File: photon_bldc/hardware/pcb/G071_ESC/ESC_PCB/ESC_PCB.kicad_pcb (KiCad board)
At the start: 6 copper layers, 12 x 32 mm, 65 parts, among them J2 Plus, J3 Minus, Q1 NMOS, Q2 NMOS, Q3 NMOS, Q4 NMOS, Q5 NMOS, Q6 NMOS, U1 STM32G071GBUx, U4 L78L06_SOT89

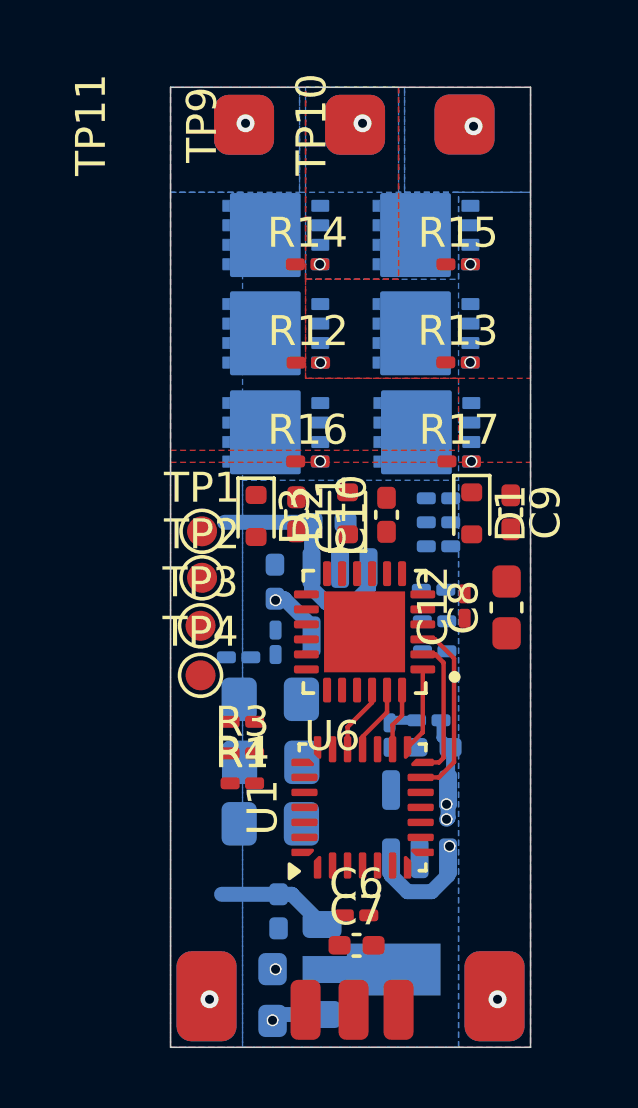
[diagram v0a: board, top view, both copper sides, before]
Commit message: ghjhbk
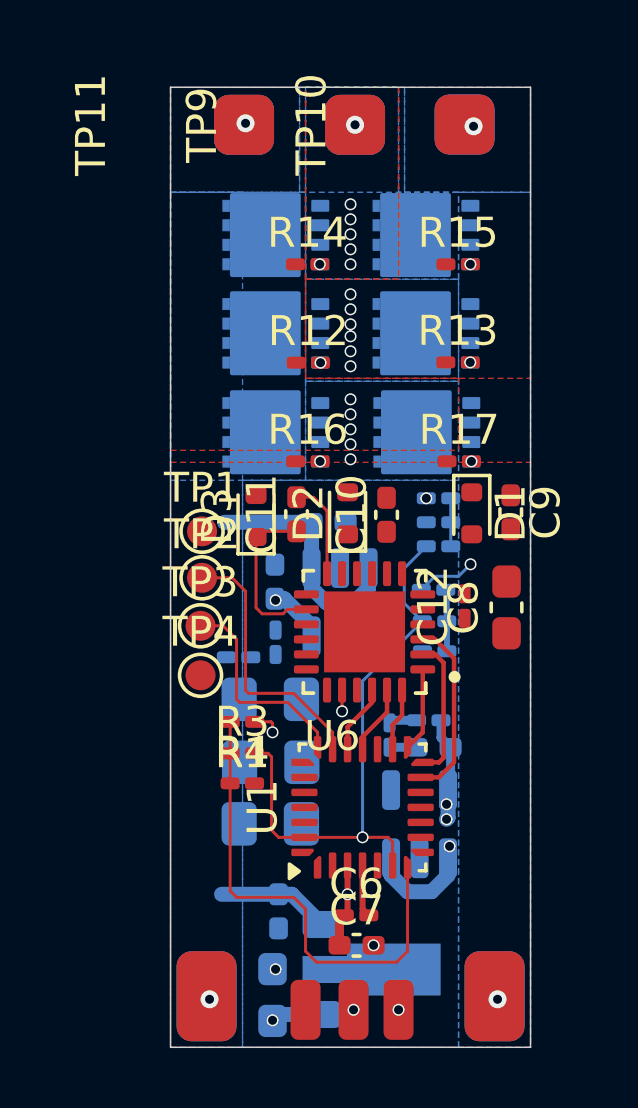
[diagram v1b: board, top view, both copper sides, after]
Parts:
- turned C11 to 90 degrees
- turned D3 to 90 degrees
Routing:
- net PHASE_C: track 0.00 -> 25.0 mm, vias 1 -> 7
- net BEMF_REF: track 0.00 -> 19.1 mm, vias 0 -> 1
- net BEMF_A: track 0.00 -> 16.3 mm
- net PHASE_A: track 0.00 -> 16.0 mm, vias 1 -> 7
- net PHASE_B: track 0.00 -> 13.1 mm, vias 1 -> 8
- net SWDIO: track 0.00 -> 8.98 mm
- net Net-(D1-K): track 0.00 -> 8.24 mm, vias 0 -> 1
- net SWCLK: track 0.00 -> 7.05 mm
- net Net-(D3-K): track 0.00 -> 5.61 mm
- net Net-(U6-VS3): track 0.00 -> 3.30 mm
- net +3.3V: track 3.53 -> 6.30 mm, vias 2 -> 3
- net GND: track 0.00 -> 2.65 mm, vias 2 -> 4
- net BEMF_C: track 0.00 -> 2.07 mm
- net BEMF_B: track 0.00 -> 1.60 mm
- net +5V: vias 1 -> 2
- added copper zone on In3.Cu, net +3.3V

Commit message: dfbdfb
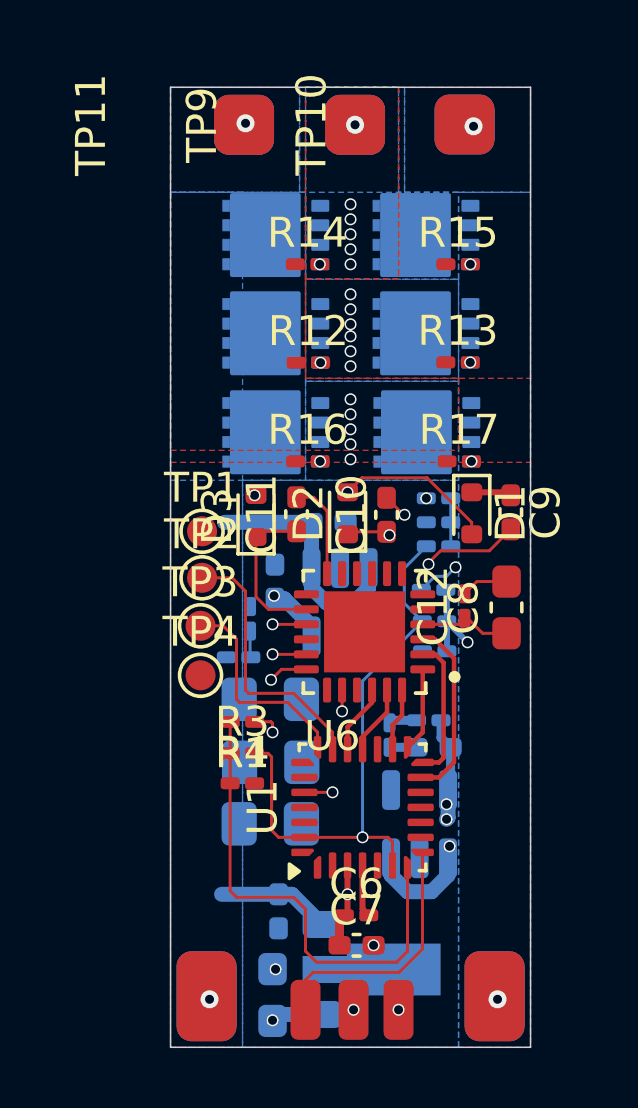
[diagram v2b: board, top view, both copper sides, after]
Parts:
- moved R19 1.16 mm to (142.7, 107.7)
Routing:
- net +6V: track 5.22 -> 16.8 mm, vias 2 -> 4
- net Net-(U6-VS1): track 0.00 -> 11.5 mm, vias 0 -> 2
- net Net-(D2-K): track 0.00 -> 10.0 mm, vias 0 -> 2
- net Net-(U6-VS2): track 0.00 -> 9.14 mm, vias 0 -> 2
- net BEMF_C: track 2.07 -> 10.9 mm, vias 0 -> 2
- net INPUT: track 0.00 -> 8.55 mm
- net GND: track 2.65 -> 4.22 mm
- net Net-(D1-K): track 8.24 -> 9.58 mm
- net ADC_VOLT: track 0.00 -> 0.89 mm
